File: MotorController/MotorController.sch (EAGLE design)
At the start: 13 parts

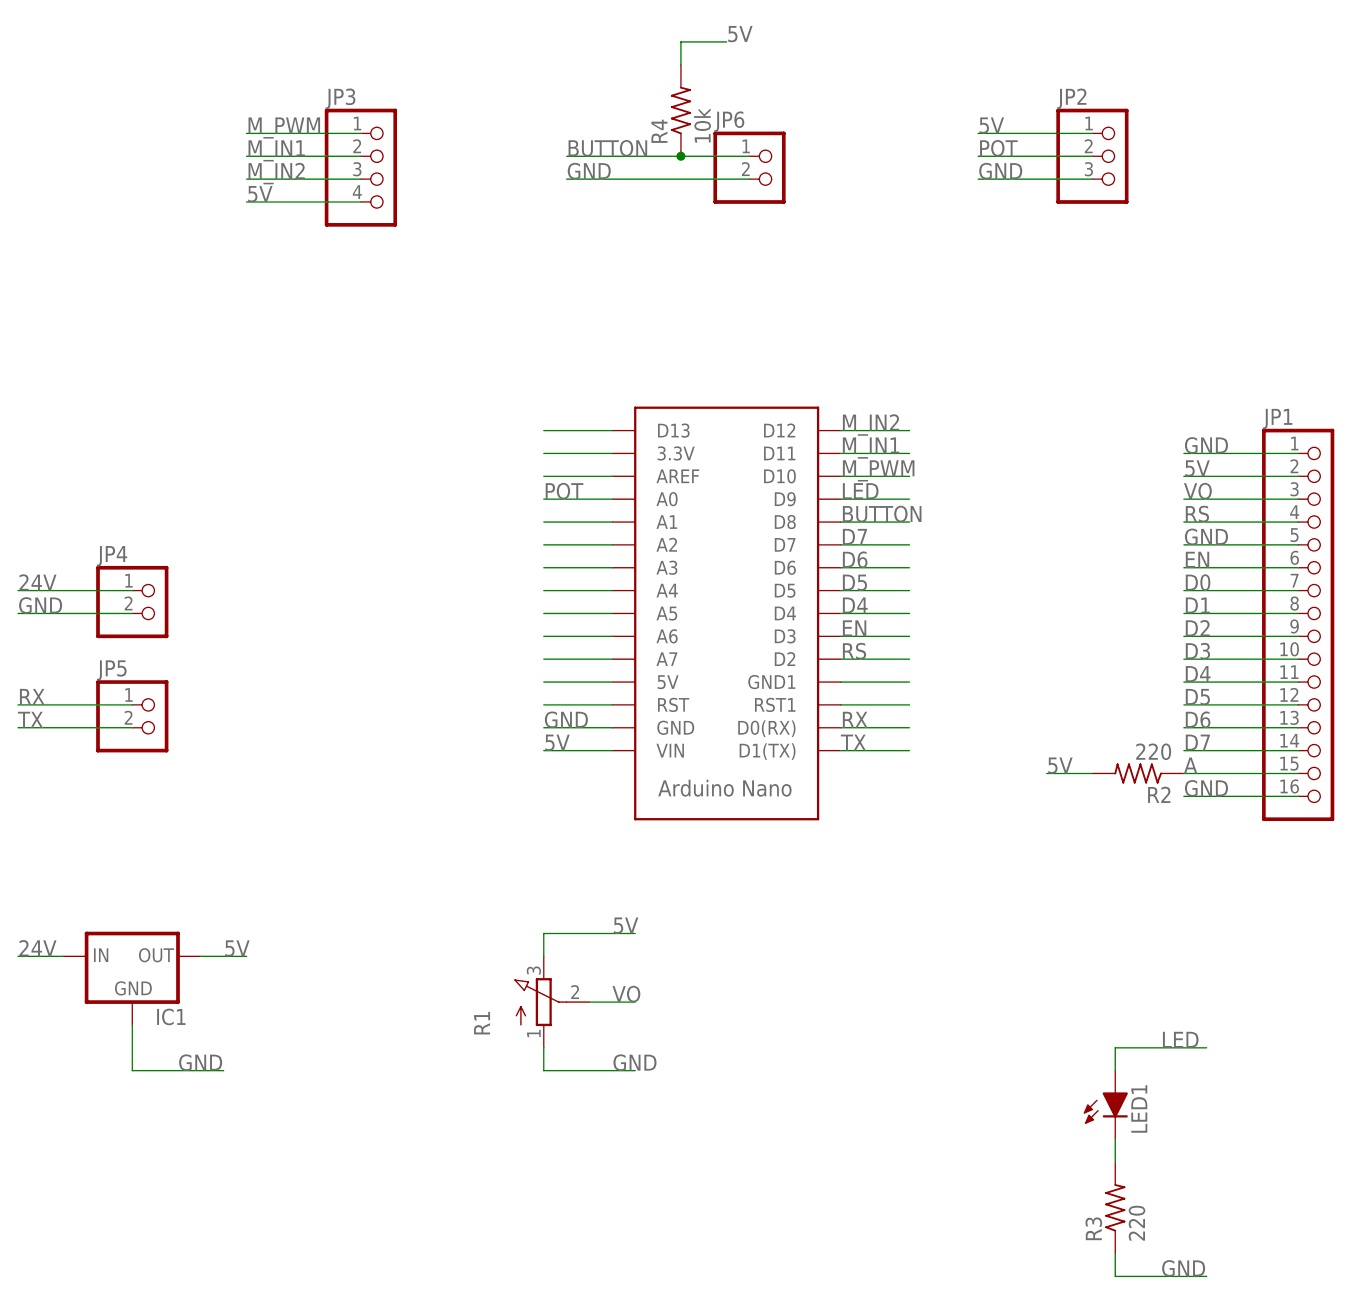
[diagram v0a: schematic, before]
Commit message: Cleaned schematics, added pdfs
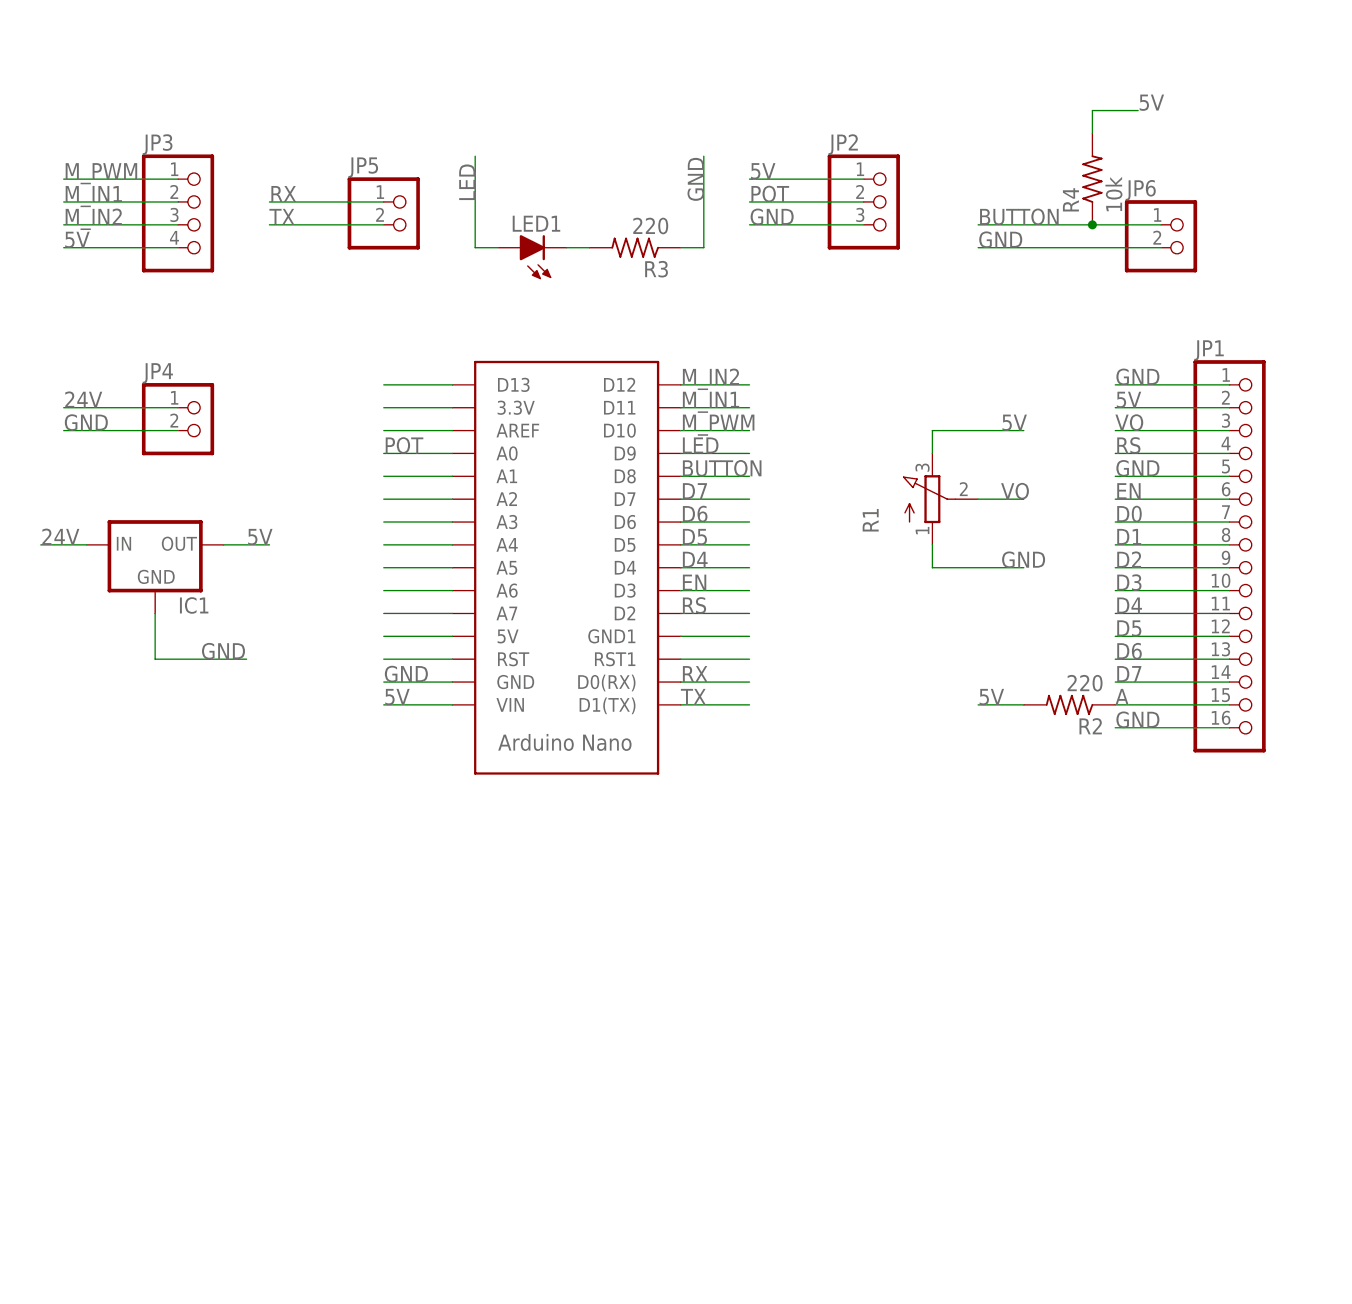
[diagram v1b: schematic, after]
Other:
- note added: "Arduino Nano"
- note added: "IO Devices"
- note added: "LCD Display"
- note added: "Motor Control"
- note added: "Power"
- moved on the sheet: IC1, JP1, JP2, JP3, JP4, JP5, JP6, LED1, R1, R2, R3, R4
